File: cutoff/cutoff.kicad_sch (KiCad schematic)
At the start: 35 parts, among them J1 Conn_01x01, J10 Conn_01x02, J11 Conn_01x01, J12 Conn_01x01, J13 Conn_01x01, J14 Conn_01x01, J15 Conn_01x01, J16 Conn_01x01, J2 Conn_01x01, J3 Conn_01x01, J4 Conn_01x01, J5 Conn_01x01, J6 Conn_01x01, J7 Conn_01x02, J8 Conn_01x01, J9 Conn_01x01, U1 TPS3700DDCR, U2 BTS50010-1TAD

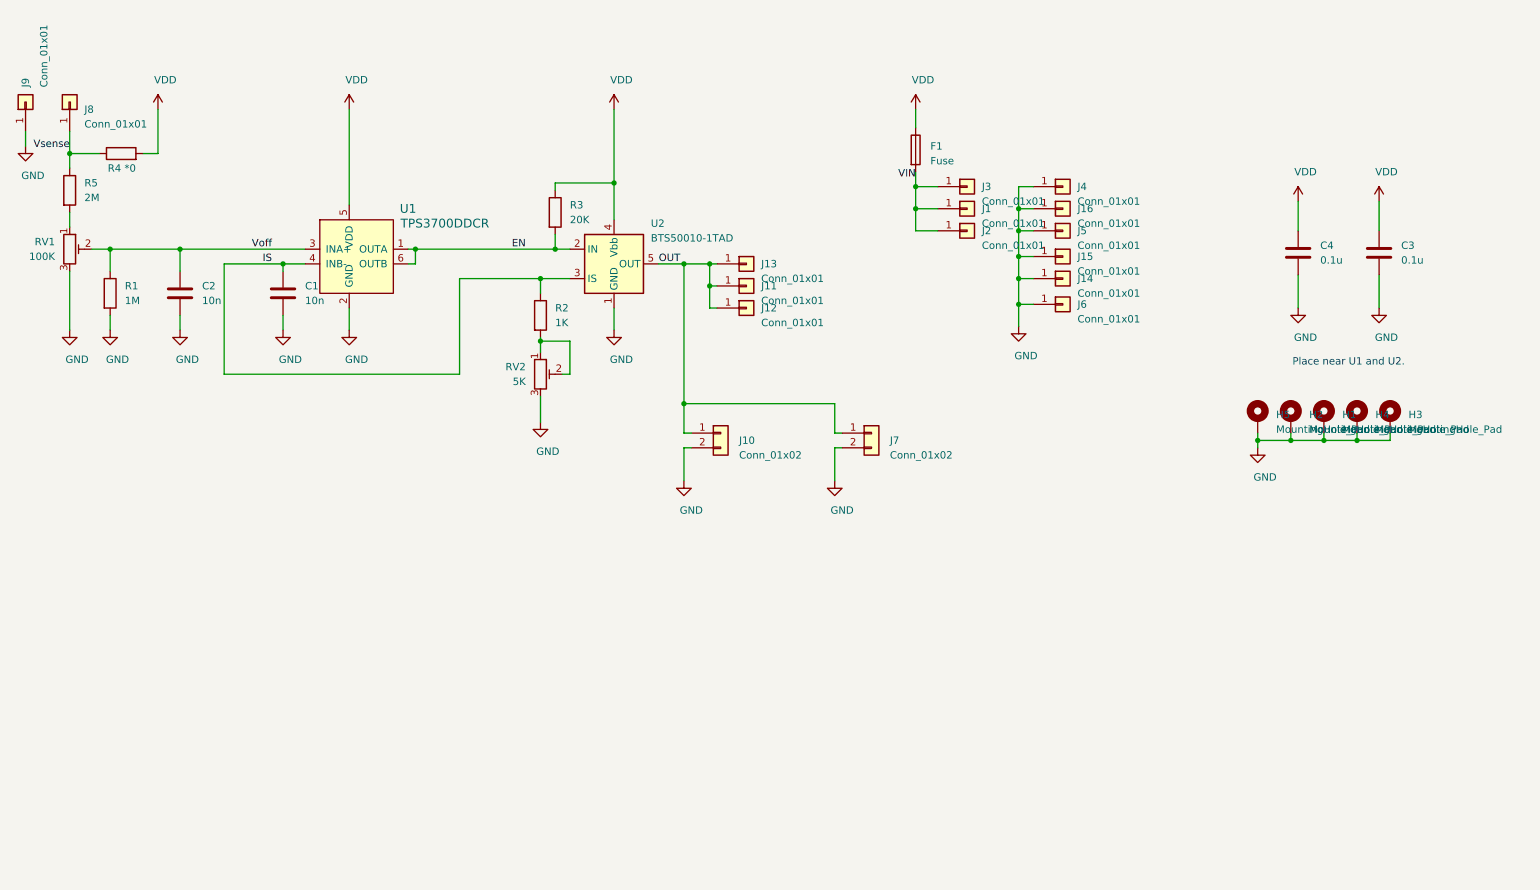
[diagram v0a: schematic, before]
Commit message: v1.1
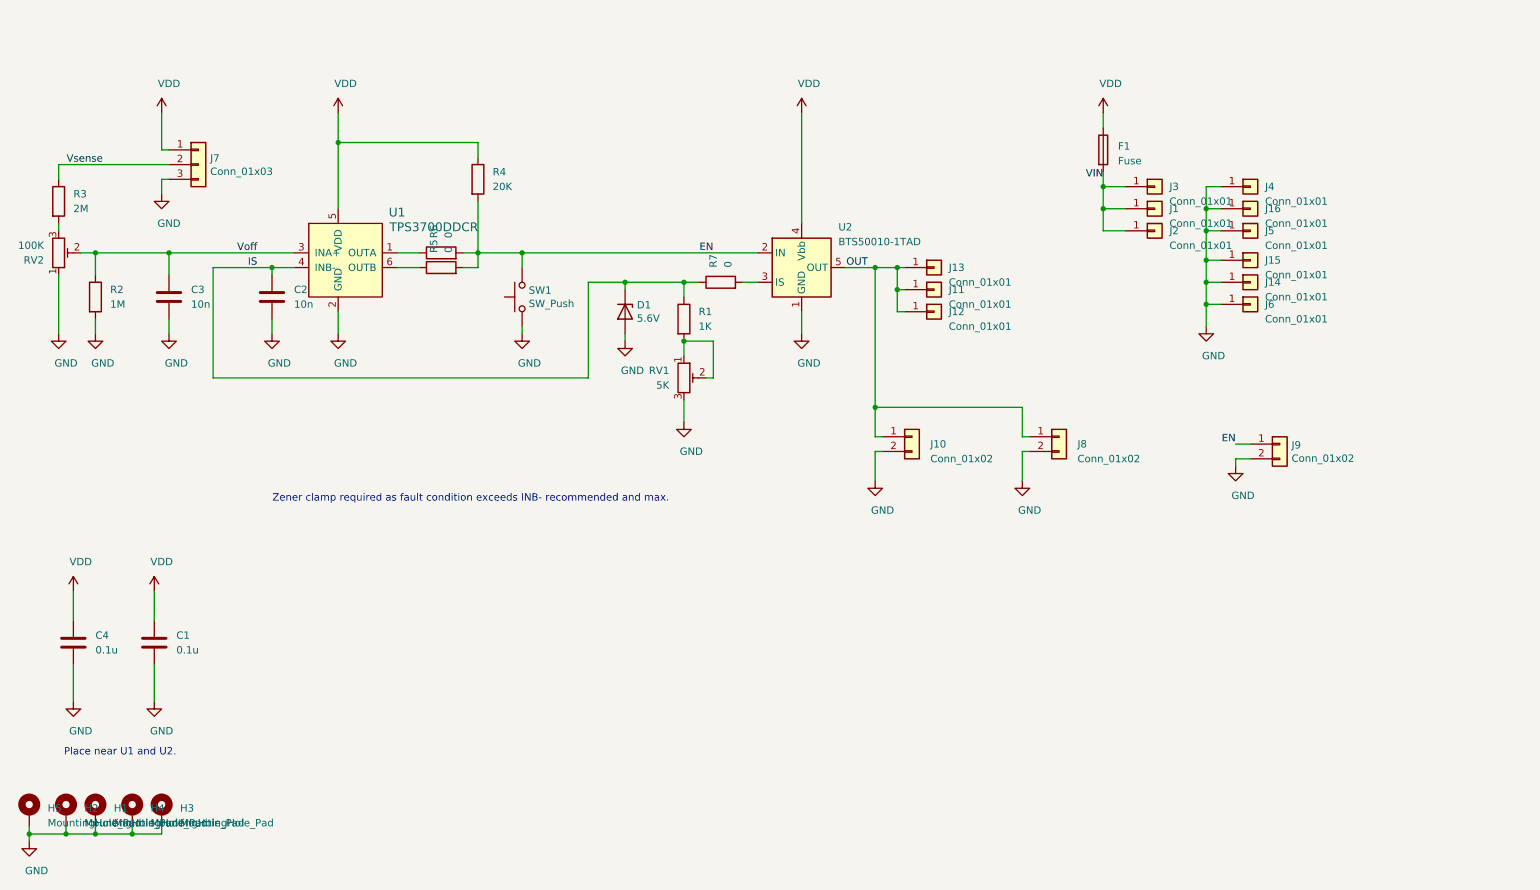
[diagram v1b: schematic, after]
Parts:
- removed J8, J9: Conn_01x01, Connector_Wire:SolderWire-0.5sqmm_1x01_D0.9mm_OD2.1mm, symbol Connector_Generic:Conn_01x01
- removed R4: *0, Resistor_SMD:R_0805_2012Metric_Pad1.20x1.40mm_HandSolder, symbol Device:R
- added D1: 5.6V, Diode_SMD:D_SOD-123, symbol Device:D_Zener
- added J7: Conn_01x03, Connector_PinHeader_2.54mm:PinHeader_1x03_P2.54mm_Vertical, symbol Connector_Generic:Conn_01x03
- added J9: Conn_01x02, Connector_PinHeader_2.54mm:PinHeader_1x02_P2.54mm_Vertical, symbol Connector_Generic:Conn_01x02
- added R5, R6, R7: 0, Resistor_SMD:R_0805_2012Metric_Pad1.20x1.40mm_HandSolder, symbol Device:R
- added SW1: SW_Push, Button_Switch_SMD:SW_SPST_PTS810, symbol Switch:SW_Push
- RV1: renamed from RV2; symbol Device:R_Potentiometer_Trim -> Device:R_POT_TRIM
- RV2: renamed from RV1; symbol Device:R_Potentiometer_Trim -> Device:R_POT_TRIM
- renumbered C3 to C1, C1 to C2, C2 to C3, J7 to J8, R2 to R1, R1 to R2, R5 to R3, R3 to R4
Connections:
- net EN: now also J9.1 (Pin_1), R5.2, R6.2, SW1.2; no longer U1.1 (OUTA), U1.6 (OUTB)
- net GND: now also RV2.1, D1.2 (A), J7.3 (Pin_3), J9.2 (Pin_2), SW1.1; no longer RV2.3
- net IS: now also D1.1 (K), R7.1; no longer U2.3 (IS)
- net VDD: now also J7.1 (Pin_1)
- net Vsense: now also J7.2 (Pin_2)
- net at R3.2: now also RV2.3; no longer RV2.1
- new net: R6.1, U1.1 (OUTA)
- new net: R7.2, U2.3 (IS)
- new net: R5.1, U1.6 (OUTB)
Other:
- note added: "Zener clamp required as fault condition exceeds INB- recommended and max."
- moved on the sheet: C1, C2, C3, C4, F1, H1, H2, H3, H4, H5, J1, J10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
